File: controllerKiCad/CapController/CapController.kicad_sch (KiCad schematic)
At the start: 1 part

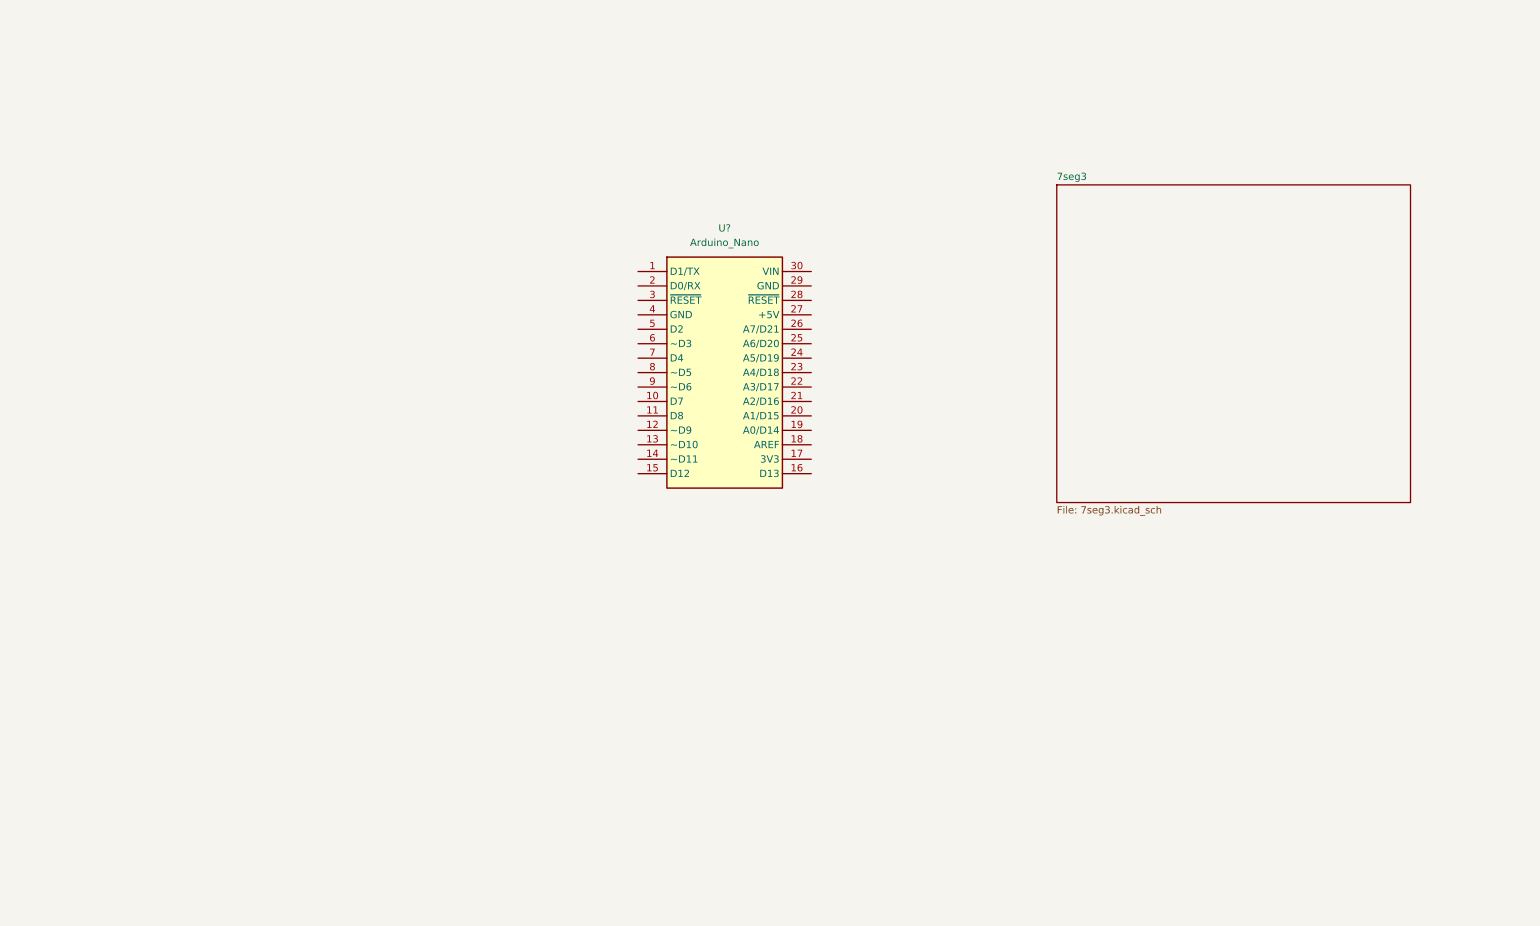
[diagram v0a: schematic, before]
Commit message: Controller PCB Update
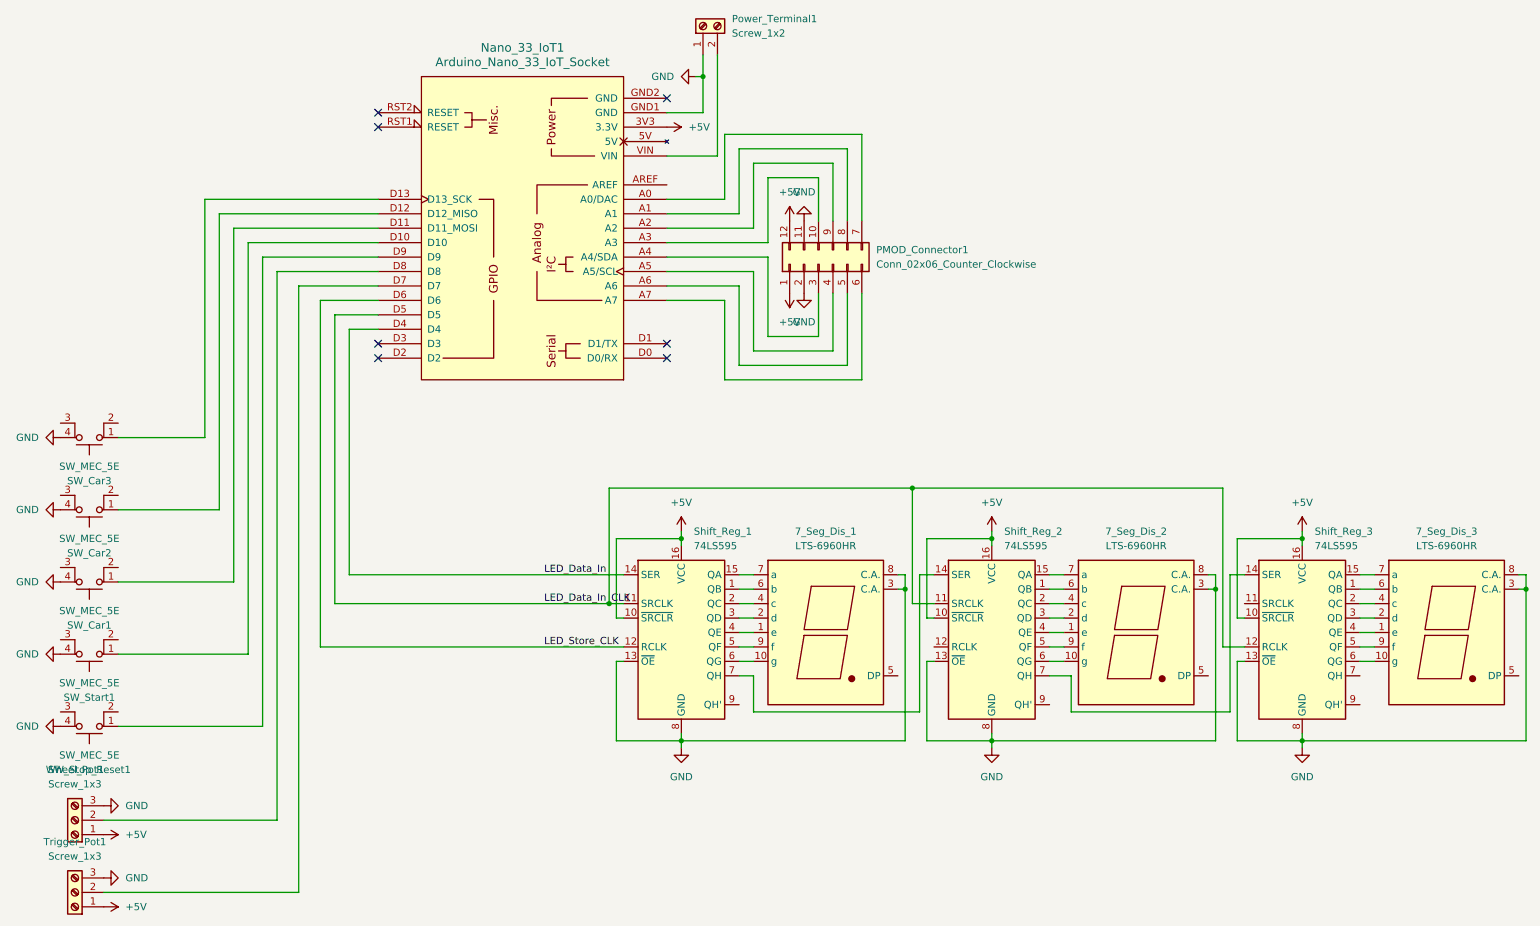
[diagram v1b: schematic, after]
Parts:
- removed U?: Arduino_Nano, Arduino:Arduino_Nano, symbol Arduino:Arduino_Nano
- added 7_Seg_Dis_1, 7_Seg_Dis_2, 7_Seg_Dis_3: LTS-6960HR, Display_7Segment:7SegmentLED_LTS6760_LTS6780, symbol Display_Character:LTS-6960HR
- added Nano_33_IoT1: Arduino_Nano_33_IoT_Socket, arduino-library:Arduino_Nano_33_IoT_Socket, symbol arduino-library:Arduino_Nano_33_IoT_Socket
- added PMOD_Connector1: Conn_02x06_Counter_Clockwise, Connector_IDC:IDC-Header_2x06_P2.54mm_Horizontal, symbol Connector_Generic:Conn_02x06_Counter_Clockwise
- added Power_Terminal1: Screw_1x2, TerminalBlock:TerminalBlock_Altech_AK300-2_P5.00mm, symbol Connector:Screw_Terminal_01x02
- added SW_Car1, SW_Car2, SW_Car3, SW_Start1, SW_Stop_Reset1: SW_MEC_5E, symbol Switch:SW_MEC_5E
- added Shift_Reg_1, Shift_Reg_2, Shift_Reg_3: 74LS595, symbol 74xx:74LS595
- added Trigger_Pot1, Wheel_Pot1: Screw_1x3, TerminalBlock:TerminalBlock_Altech_AK300-3_P5.00mm, symbol Connector:Screw_Terminal_01x03
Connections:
- new net: Nano_33_IoT1.D8, Wheel_Pot1.2 (Pin_2)
- new net: Nano_33_IoT1.D13 (D13_SCK), SW_Car3.1
- new net: Nano_33_IoT1.D12 (D12_MISO), SW_Car2.1
- new net: Nano_33_IoT1.VIN, Power_Terminal1.2 (Pin_2)
- new net: 7_Seg_Dis_3.1 (e), Shift_Reg_3.4 (QE)
- new net: 7_Seg_Dis_3.10 (g), Shift_Reg_3.6 (QG)
- new net: 7_Seg_Dis_3.2 (d), Shift_Reg_3.3 (QD)
- new net: 7_Seg_Dis_3.4 (c), Shift_Reg_3.2 (QC)
- new net: 7_Seg_Dis_3.6 (b), Shift_Reg_3.1 (QB)
- new net: 7_Seg_Dis_3.7 (a), Shift_Reg_3.15 (QA)
- new net: 7_Seg_Dis_3.9 (f), Shift_Reg_3.5 (QF)
- new net: Nano_33_IoT1.D10, SW_Start1.1
- new net: 7_Seg_Dis_2.1 (e), Shift_Reg_2.4 (QE)
- new net: 7_Seg_Dis_2.10 (g), Shift_Reg_2.6 (QG)
- new net: 7_Seg_Dis_2.2 (d), Shift_Reg_2.3 (QD)
- new net: 7_Seg_Dis_2.4 (c), Shift_Reg_2.2 (QC)
- new net: 7_Seg_Dis_2.6 (b), Shift_Reg_2.1 (QB)
- new net: 7_Seg_Dis_2.7 (a), Shift_Reg_2.15 (QA)
- new net: 7_Seg_Dis_2.9 (f), Shift_Reg_2.5 (QF)
- new net: Nano_33_IoT1.A3, PMOD_Connector1.10 (Pin_10)
- new net: Nano_33_IoT1.A4 (A4/SDA), PMOD_Connector1.3 (Pin_3)
- new net: Nano_33_IoT1.A5 (A5/SCL), PMOD_Connector1.4 (Pin_4)
- new net: Nano_33_IoT1.A6, PMOD_Connector1.5 (Pin_5)
- new net: Nano_33_IoT1.A7, PMOD_Connector1.6 (Pin_6)
- new net: Nano_33_IoT1.A0 (A0/DAC), PMOD_Connector1.7 (Pin_7)
- new net: Nano_33_IoT1.A1, PMOD_Connector1.8 (Pin_8)
- new net: Nano_33_IoT1.A2, PMOD_Connector1.9 (Pin_9)
- new net: Shift_Reg_1.7 (QH), Shift_Reg_2.14 (SER)
- new net: Shift_Reg_2.7 (QH), Shift_Reg_3.14 (SER)
- new net: Nano_33_IoT1.D11 (D11_MOSI), SW_Car1.1
- new net: Nano_33_IoT1.D7, Trigger_Pot1.2 (Pin_2)
- new net: Nano_33_IoT1.D9, SW_Stop_Reset1.1
- new net: 7_Seg_Dis_1.6 (b), Shift_Reg_1.1 (QB)
- new net: 7_Seg_Dis_1.7 (a), Shift_Reg_1.15 (QA)
- new net: 7_Seg_Dis_1.4 (c), Shift_Reg_1.2 (QC)
- new net: 7_Seg_Dis_1.2 (d), Shift_Reg_1.3 (QD)
- new net: 7_Seg_Dis_1.1 (e), Shift_Reg_1.4 (QE)
- new net: 7_Seg_Dis_1.9 (f), Shift_Reg_1.5 (QF)
- new net: 7_Seg_Dis_1.10 (g), Shift_Reg_1.6 (QG)
- new net +5V: Nano_33_IoT1.3V3 (3.3V), PMOD_Connector1.1 (Pin_1), PMOD_Connector1.12 (Pin_12), Shift_Reg_1.10 (~{SRCLR}), Shift_Reg_1.16 (VCC), Shift_Reg_2.10 (~{SRCLR}), Shift_Reg_2.16 (VCC), Shift_Reg_3.10 (~{SRCLR}), Shift_Reg_3.16 (VCC), Trigger_Pot1.1 (Pin_1), Wheel_Pot1.1 (Pin_1)
- new net GND: 7_Seg_Dis_1.3 (C.A.), 7_Seg_Dis_1.8 (C.A.), 7_Seg_Dis_2.3 (C.A.), 7_Seg_Dis_2.8 (C.A.), 7_Seg_Dis_3.3 (C.A.), 7_Seg_Dis_3.8 (C.A.), Nano_33_IoT1.GND1 (GND), PMOD_Connector1.11 (Pin_11), PMOD_Connector1.2 (Pin_2), Power_Terminal1.1 (Pin_1), SW_Car1.4 (A), SW_Car2.4 (A), SW_Car3.4 (A), SW_Start1.4 (A), SW_Stop_Reset1.4 (A), Shift_Reg_1.13 (~{OE}), Shift_Reg_1.8 (GND), Shift_Reg_2.13 (~{OE}), Shift_Reg_2.8 (GND), Shift_Reg_3.13 (~{OE}), Shift_Reg_3.8 (GND), Trigger_Pot1.3 (Pin_3), Wheel_Pot1.3 (Pin_3)
- new net LED_Data_In: Nano_33_IoT1.D4, Shift_Reg_1.14 (SER)
- new net LED_Data_In_CLK: Nano_33_IoT1.D5, Shift_Reg_1.11 (SRCLK), Shift_Reg_2.11 (SRCLK), Shift_Reg_3.12 (RCLK)
- new net LED_Store_CLK: Nano_33_IoT1.D6, Shift_Reg_1.12 (RCLK)
- no-connect marks 0 -> 7
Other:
- removed sheet 7seg3
